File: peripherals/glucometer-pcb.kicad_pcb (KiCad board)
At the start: 2 copper layers, 46.3 x 68 mm, 12 parts, among them U1 ESP32_DevKit_V1_DOIT

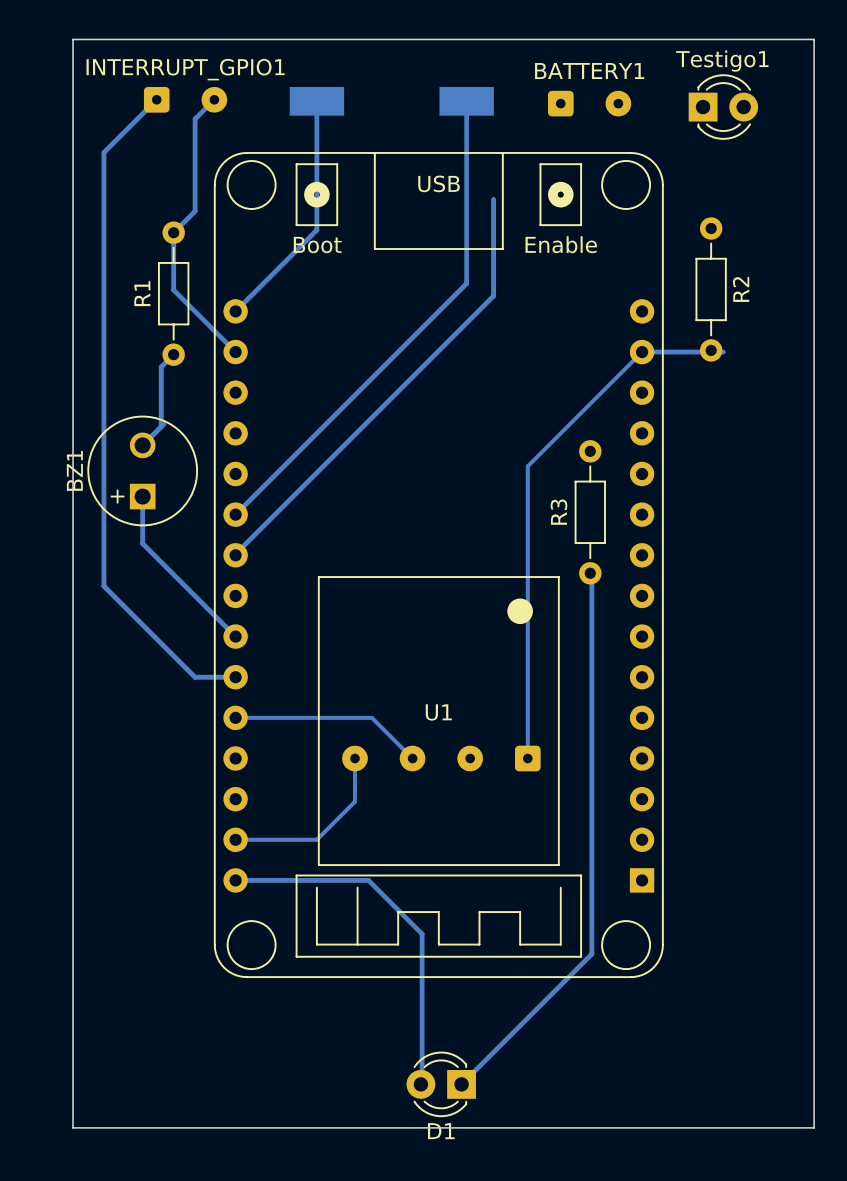
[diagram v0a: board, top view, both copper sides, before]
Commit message: last update emmiter pcb
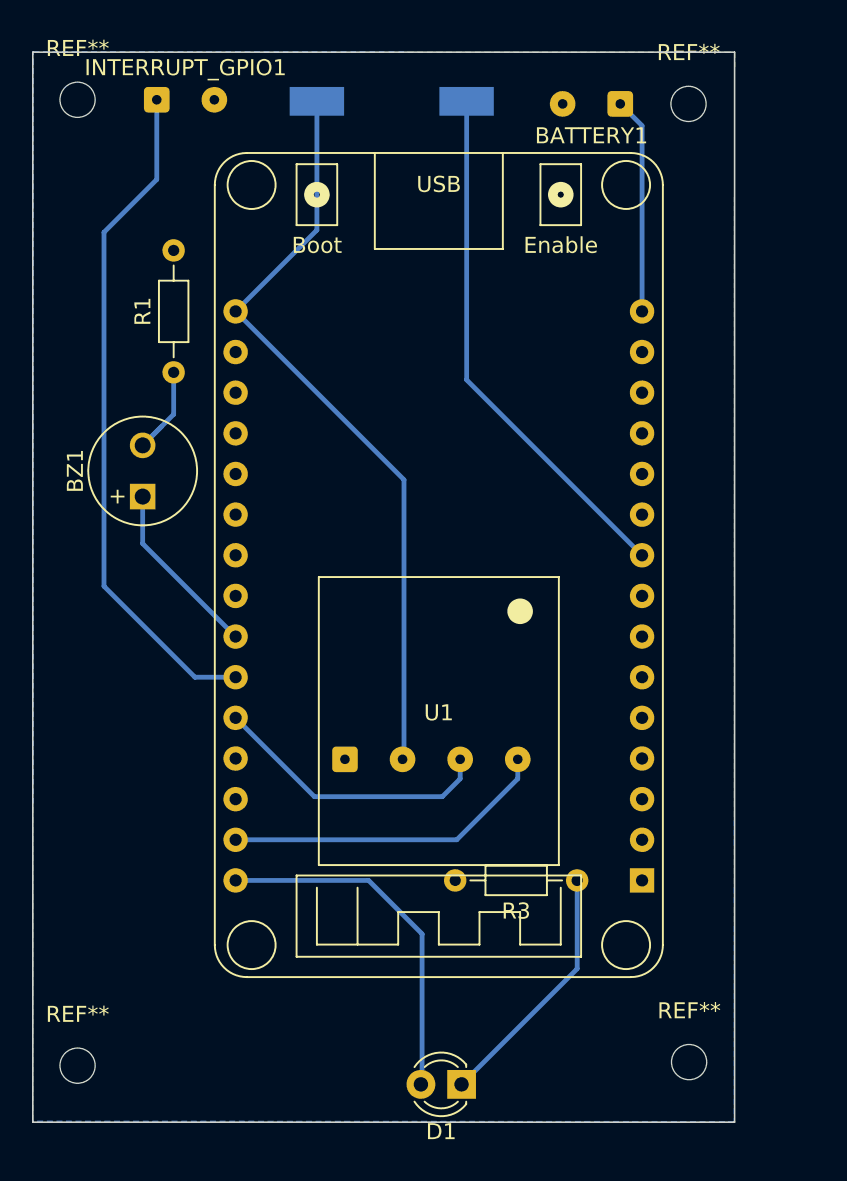
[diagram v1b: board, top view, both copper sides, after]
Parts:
- removed R2: 120, Resistor_THT:R_Axial_DIN0204_L3.6mm_D1.6mm_P7.62mm_Horizontal
- removed Testigo1: LED, LED_THT:LED_D3.0mm_FlatTop
- added REF**: MountingHole_2.2mm_M2, MountingHole:MountingHole_2.2mm_M2, F.Cu at (185.7, 131.0)
- added REF**: MountingHole_2.2mm_M2, MountingHole:MountingHole_2.2mm_M2, F.Cu at (223.9, 130.7)
- added REF**: MountingHole_2.2mm_M2, MountingHole:MountingHole_2.2mm_M2, F.Cu at (185.7, 70.6)
- added REF**: MountingHole_2.2mm_M2, MountingHole:MountingHole_2.2mm_M2, F.Cu at (223.9, 70.9)
- moved R3 19.2 mm to (216.9, 119.4), turned to 180 degrees
- moved BATTERY1 3.72 mm to (219.6, 70.9), turned to 180 degrees
- moved OLED_PINS1 1.27 mm to (212.6, 111.8)
- moved R1 1.11 mm to (191.7, 87.6)
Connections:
- net VCC renamed Net-(3V3_OUT1-Pad1)
- U1 pad 21: Net-(SIGNAL_IN1-Pad1) -> unconnected-(U1-Pad21)
- U1 pad 8: Net-(U1-Pad8) -> unconnected-(U1-Pad8)
- U1 pad 9: unconnected-(U1-Pad9) -> Net-(SIGNAL_IN1-Pad1)
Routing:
- net GND: track 51.9 -> 0.09 mm
- net Net-(3V3_OUT1-Pad1): track 15.2 -> 47.6 mm
- net unconnected-(U1-Pad22): track 28.9 -> 0.00 mm
- net Net-(D1-Pad1): track 35.4 -> 15.7 mm
- net Net-(BATTERY1-Pad1): track 0.00 -> 13.5 mm
- net Net-(OLED_PINS1-Pad4): track 11.1 -> 20.4 mm
- net Net-(OLED_PINS1-Pad3): track 12.1 -> 17.8 mm
- net Net-(BZ1-Pad2): track 8.35 -> 7.00 mm
- added copper zone on B.Cu, net GND
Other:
- board size 46.3 x 68 mm -> 43.9 x 66.9 mm
